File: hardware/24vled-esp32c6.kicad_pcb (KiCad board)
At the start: 2 copper layers, 67 x 84.5 mm, 5 parts, among them J1 Conn_01x20, J2 Conn_01x20, J3 Barrel_Jack, J5 2604-1106, U1 LM2596S-5

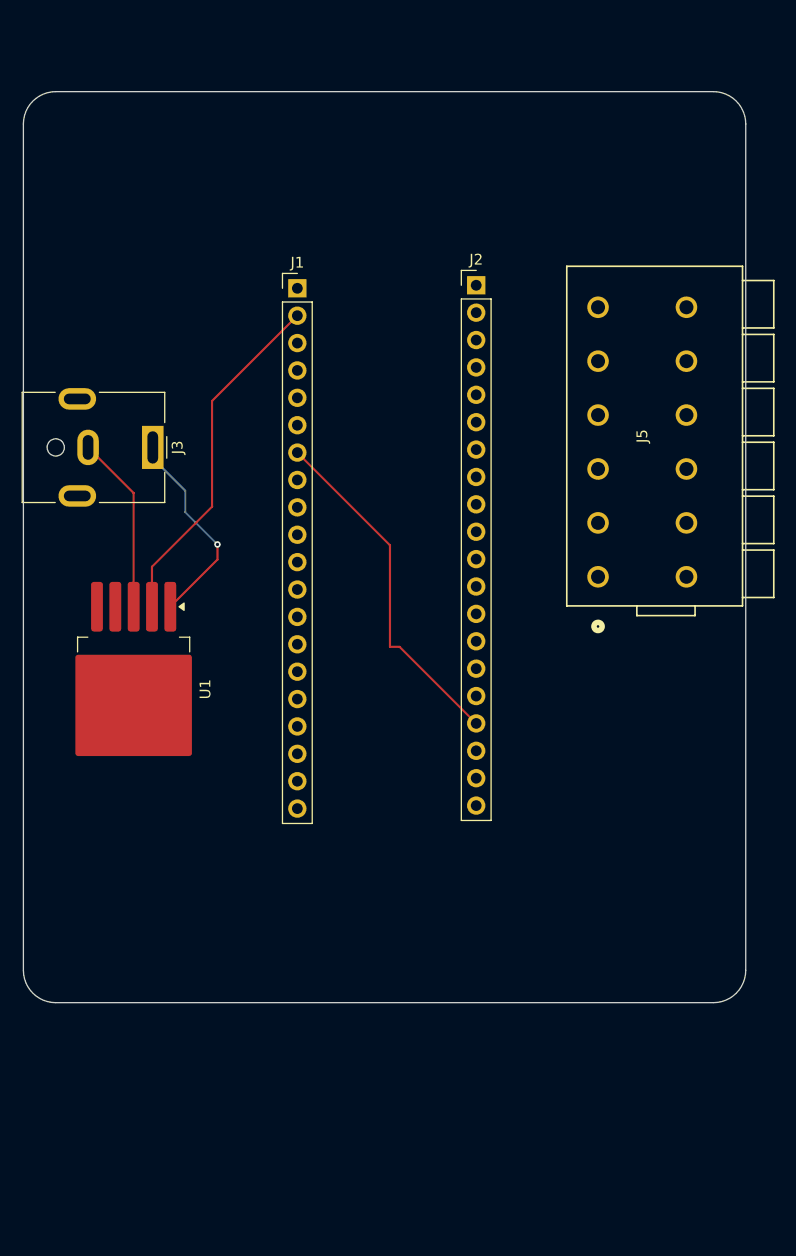
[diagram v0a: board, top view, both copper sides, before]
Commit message: hardware v1
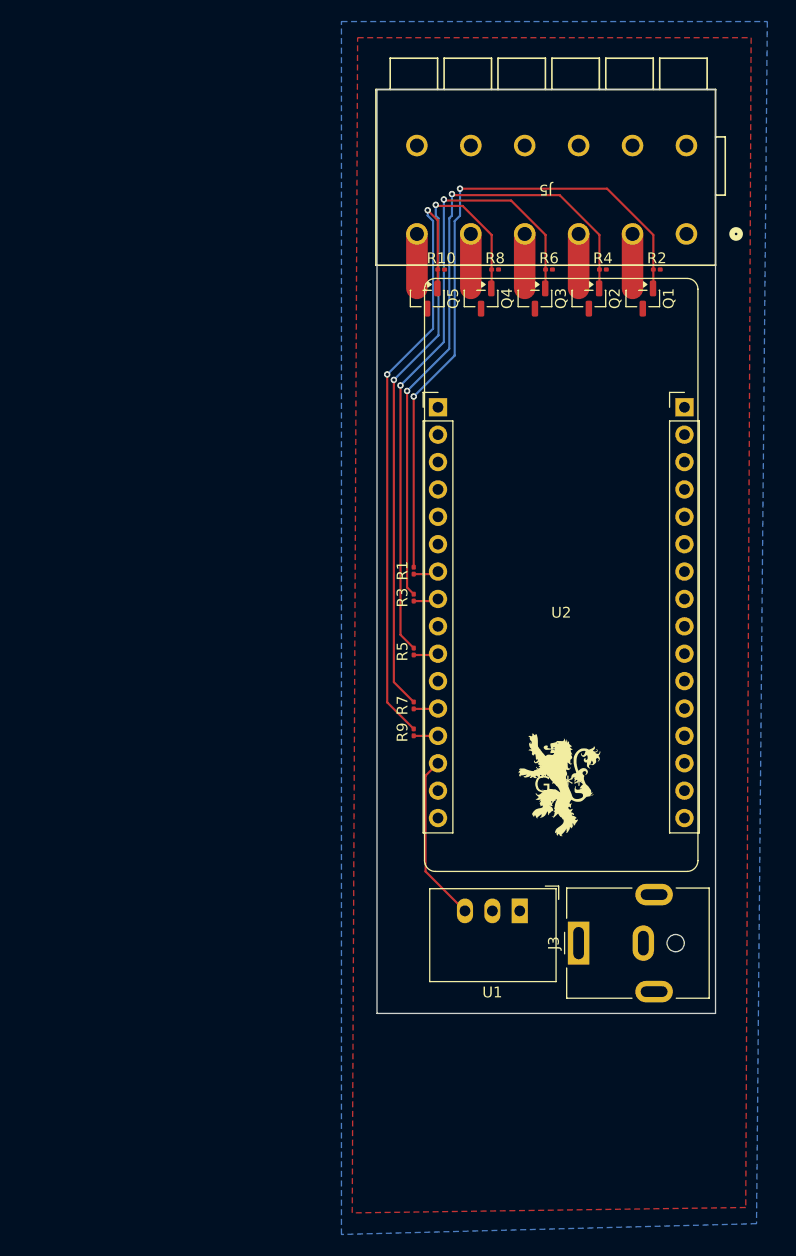
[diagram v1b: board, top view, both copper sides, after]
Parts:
- removed J1, J2: Conn_01x20, Connector_PinHeader_2.54mm:PinHeader_1x20_P2.54mm_Vertical
- added G***: LOGO, Library:industries_10mm, F.Cu at (152.2, 104.3)
- added Q1: AO3400A, Package_TO_SOT_SMD:SOT-23, F.Cu at (159.9, 59.2)
- added Q2: AO3400A, Package_TO_SOT_SMD:SOT-23, F.Cu at (154.9, 59.2)
- added Q3: AO3400A, Package_TO_SOT_SMD:SOT-23, F.Cu at (149.9, 59.2)
- added Q4: AO3400A, Package_TO_SOT_SMD:SOT-23, F.Cu at (144.9, 59.2)
- added Q5: AO3400A, Package_TO_SOT_SMD:SOT-23, F.Cu at (139.9, 59.2)
- added R1: 100, Resistor_SMD:R_0201_0603Metric, F.Cu at (138.7, 84.4)
- added R10: 10k, Resistor_SMD:R_0201_0603Metric, F.Cu at (141.2, 56.5)
- added R2: 10k, Resistor_SMD:R_0201_0603Metric, F.Cu at (161.2, 56.5)
- added R3: 100, Resistor_SMD:R_0201_0603Metric, F.Cu at (138.7, 86.9)
- added R4: 10k, Resistor_SMD:R_0201_0603Metric, F.Cu at (156.2, 56.5)
- added R5: 100, Resistor_SMD:R_0201_0603Metric, F.Cu at (138.7, 91.9)
- added R6: 10k, Resistor_SMD:R_0201_0603Metric, F.Cu at (151.2, 56.5)
- added R7: 100, Resistor_SMD:R_0201_0603Metric, F.Cu at (138.7, 96.9)
- added R8: 10k, Resistor_SMD:R_0201_0603Metric, F.Cu at (146.2, 56.5)
- added R9: 100, Resistor_SMD:R_0201_0603Metric, F.Cu at (138.7, 99.4)
- added U2: ~, Library:Waveshare ESP32c6, F.Cu at (152.4, 88.8)
- U1: value LM2596S-5 -> R-78E5.0-1.0; footprint Package_TO_SOT_SMD:TO-263-5_TabPin3 -> Converter_DCDC:Converter_DCDC_RECOM_R-78E-0.5_THT
- moved J3 60.6 mm to (154.0, 119.0), turned to 90 degrees
- moved U1 41.3 mm to (148.5, 116.0), turned to 180 degrees
- moved J5 32.8 mm to (164.0, 53.2), turned to 180 degrees
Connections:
- J3 pad 1: Net-(U1-VIN) -> +24V
- J3 pad 2: Net-(U1-GND) -> GND
- J5 pad 1: unconnected-(J5-1_1-Pad1) -> +24V
- J5 pad 11: unconnected-(J5-6_1-Pad11) -> WW24
- J5 pad 3: unconnected-(J5-2_1-Pad3) -> R24
- J5 pad 5: unconnected-(J5-3_1-Pad5) -> G24
- J5 pad 7: unconnected-(J5-4_1-Pad7) -> B24
- J5 pad 9: unconnected-(J5-5_1-Pad9) -> CW24
- U1 pad 1: Net-(U1-VIN) -> +24V
- U1 pad 2: +5V -> GND
- U1 pad 3: Net-(U1-GND) -> +5V
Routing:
- net Net-(Q1-G): track 0.00 -> 61.6 mm, vias 0 -> 2
- net Net-(Q4-G): track 0.00 -> 60.1 mm, vias 0 -> 2
- net Net-(Q3-G): track 0.00 -> 59.6 mm, vias 0 -> 2
- net Net-(Q2-G): track 0.00 -> 59.4 mm, vias 0 -> 2
- net Net-(Q5-G): track 0.00 -> 58.8 mm, vias 0 -> 2
- net (no net): track 32.5 -> 0.00 mm
- net Net-(U1-VIN): track 19.1 -> 0.00 mm, vias 1 -> 0
- net +5V: track 32.6 -> 15.7 mm
- net Net-(U1-GND): track 16.5 -> 0.00 mm
- net WW24: track 0.00 -> 5.05 mm
- net R24: track 0.00 -> 5.05 mm
- net G24: track 0.00 -> 5.05 mm
- net CW24: track 0.00 -> 5.05 mm
- net B24: track 0.00 -> 5.05 mm
- net R3.3: track 0.00 -> 2.72 mm
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- added copper zone on B.Cu, net +24V
- added copper zone on F.Cu, net GND
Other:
- board size 67 x 84.5 mm -> 31.4 x 85.7 mm

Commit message: hardware v2
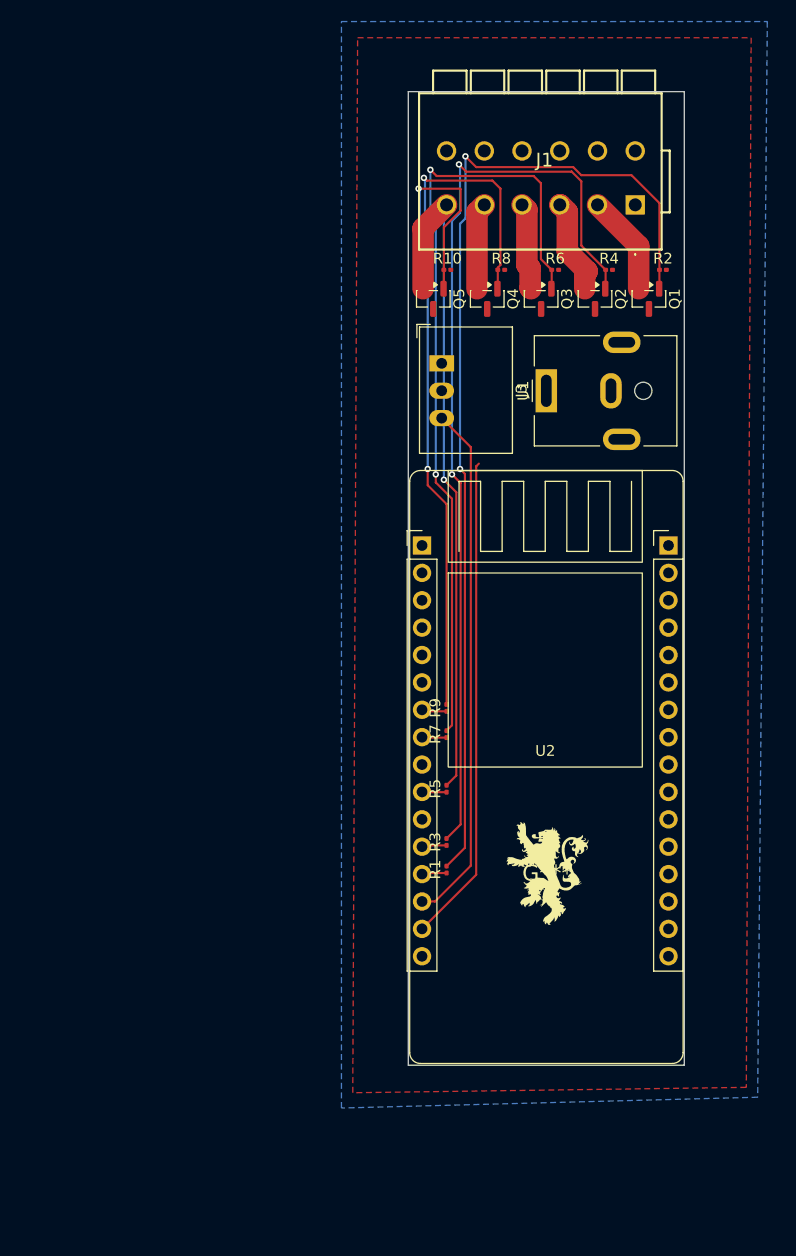
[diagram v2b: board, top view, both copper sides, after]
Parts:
- removed J5: 2604-1106, Wago:CONN6_2604-1106_WAG
- added J1: 2601-1106, External:26011106, F.Cu at (159.2, 50.5)
- moved J3 51.3 mm to (151.0, 67.8)
- moved U1 51.3 mm to (141.3, 65.2), turned to -90 degrees
- moved R1 27.9 mm to (141.8, 112.2)
- moved R3 22.9 mm to (141.8, 109.6)
- moved R5 13.1 mm to (141.8, 104.7)
- moved U2 12.9 mm to (150.9, 101.6)
- moved G*** 8.30 mm to (151.1, 112.5)
- moved R7 4.05 mm to (141.8, 99.6)
- moved R9 3.80 mm to (141.8, 97.2)
- moved Q1 0.57 mm to (160.5, 59.2)
- moved Q2 0.57 mm to (155.5, 59.2)
- moved Q3 0.57 mm to (150.5, 59.2)
- moved Q4 0.57 mm to (145.5, 59.2)
- moved Q5 0.57 mm to (140.5, 59.2)
- moved R10 0.57 mm to (141.8, 56.5)
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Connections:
- U2 pad 12: CW3.3 -> G3.3
- U2 pad 13: WW3.3 -> R3.3
- U2 pad 7: R3.3 -> WW3.3
- U2 pad 8: G3.3 -> CW3.3
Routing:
- net GND: track 0.00 -> 45.3 mm
- net Net-(Q1-G): track 61.6 -> 94.7 mm
- net +5V: track 15.7 -> 48.5 mm
- net Net-(Q2-G): track 59.4 -> 86.7 mm
- net Net-(Q3-G): track 59.6 -> 79.4 mm
- net Net-(Q4-G): track 60.1 -> 69.5 mm
- net R24: track 5.05 -> 9.36 mm
- net Net-(Q5-G): track 58.8 -> 62.8 mm
- net G24: track 5.05 -> 8.96 mm
- net WW24: track 5.05 -> 8.83 mm
- net B24: track 5.05 -> 8.12 mm
- net CW24: track 5.05 -> 8.06 mm
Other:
- board size 31.4 x 85.7 mm -> 25.6 x 90.3 mm
